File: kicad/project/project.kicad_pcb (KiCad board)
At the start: 2 copper layers, 98 x 60 mm, 42 parts, among them J1 SWD, J3 Voltmeter, U1 ADS1015, U2 AP7380, U3 STM32L031F4Px, U4 VN7003ALH

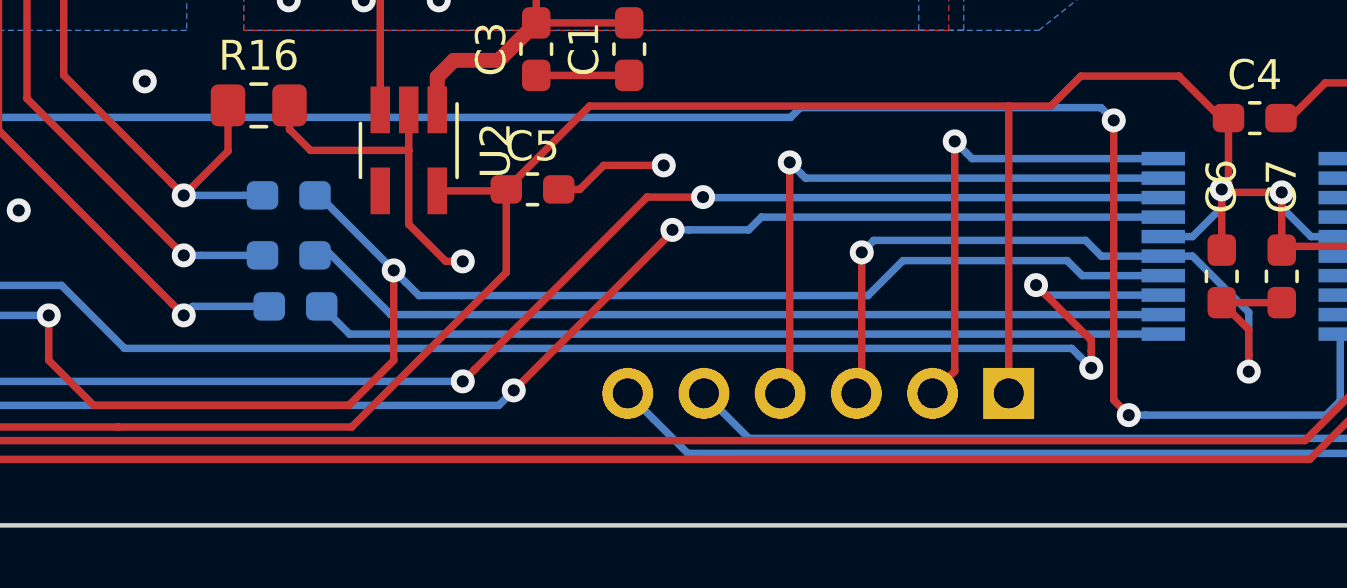
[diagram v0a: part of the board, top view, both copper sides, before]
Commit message: Solder mask
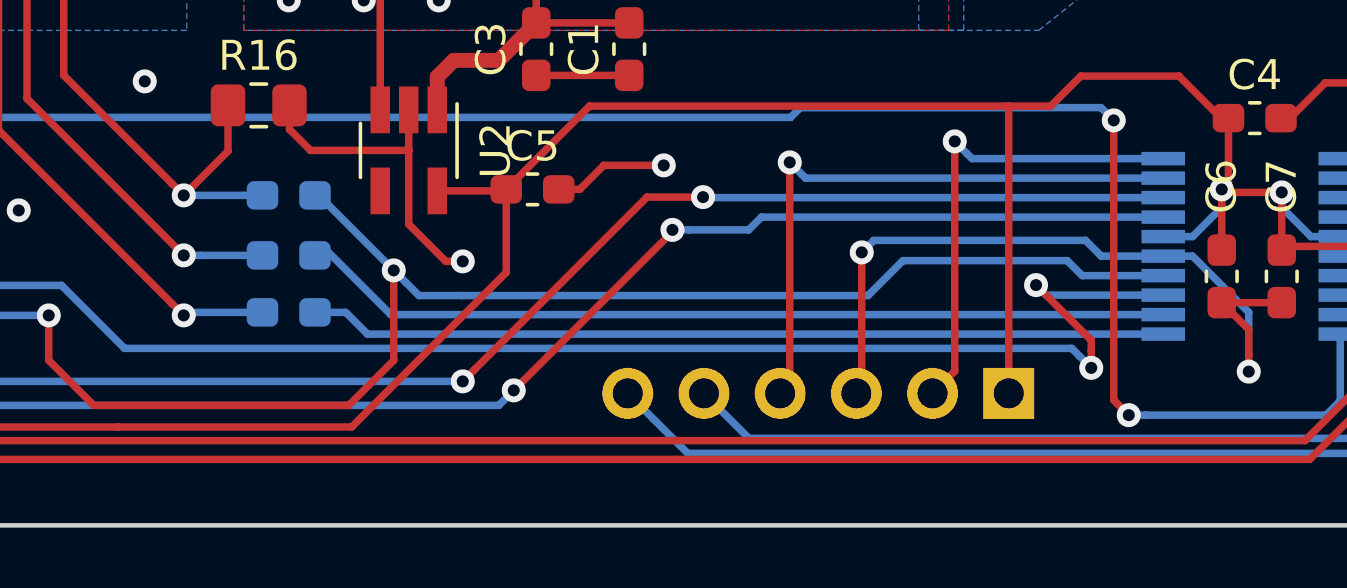
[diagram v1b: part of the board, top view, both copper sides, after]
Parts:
- moved R11 0.30 mm to (137.5, 127.9)
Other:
- rule pad_to_mask_clearance: 0.051 -> 0
